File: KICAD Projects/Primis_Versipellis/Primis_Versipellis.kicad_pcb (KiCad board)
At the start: 2 copper layers, 50 x 26 mm, 29 parts, among them J2 USB_A, J3 Conn_01x05_Pin, U1 nRF52833_QDxx, Y2 Crystal_GND24

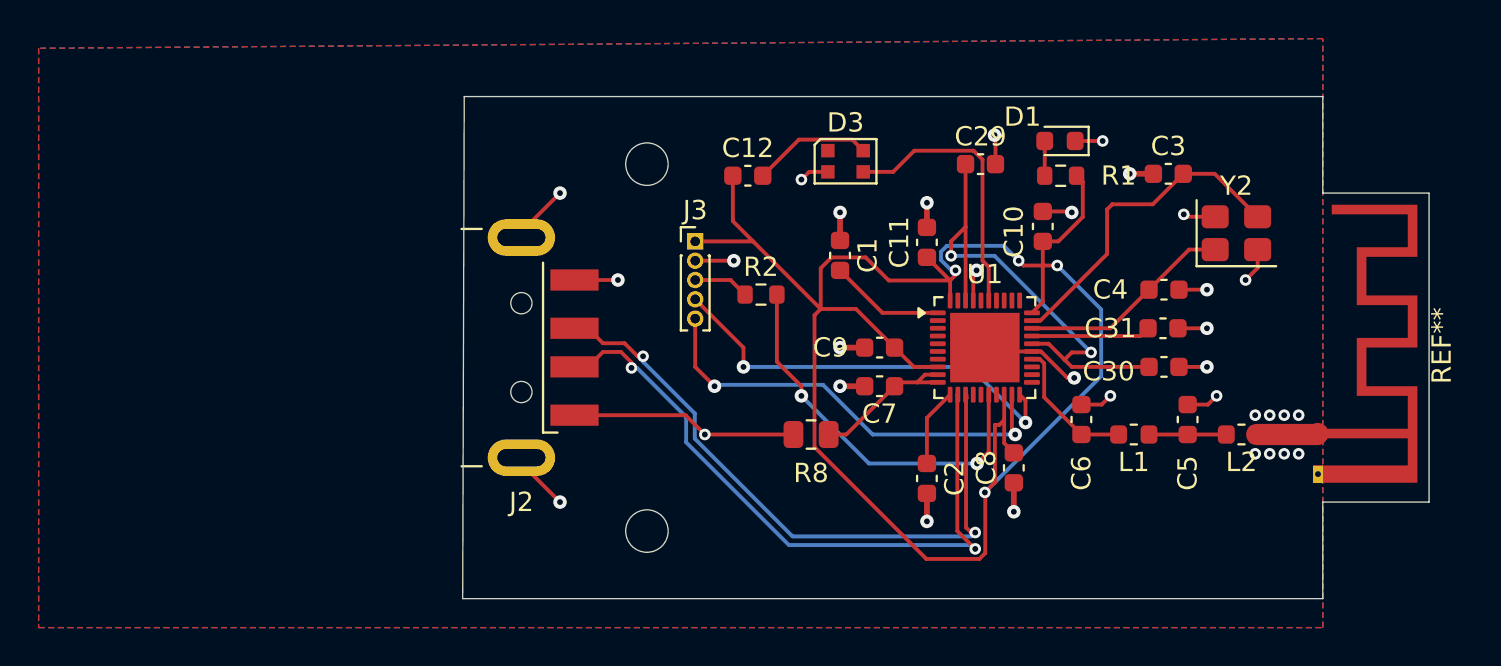
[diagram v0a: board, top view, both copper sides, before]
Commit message: Usb swap
-Changed the dongle to another usb
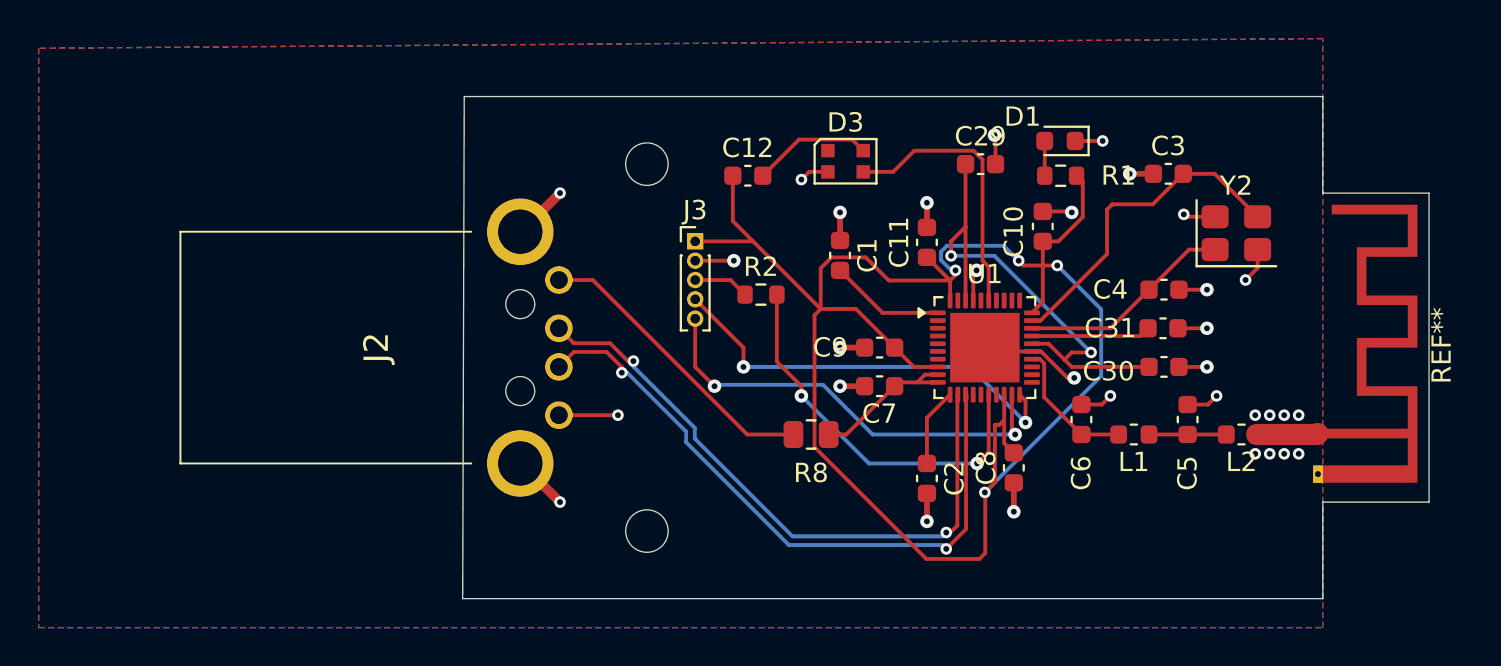
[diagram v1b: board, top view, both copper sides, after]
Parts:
- J2: footprint Connector_USB:USB_A_CNCTech_1001-011-01101_Horizontal -> USB:USB05
- moved J2 9.51 mm to (129.4, 66.0), turned to -90 degrees
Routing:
- net VBUS: track 12.1 -> 15.7 mm, vias 1 -> 0
- net D-: track 34.6 -> 32.6 mm
